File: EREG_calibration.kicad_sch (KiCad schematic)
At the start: 22 parts, among them T1 Low pressure water tank, T2 High pressure COTS tank

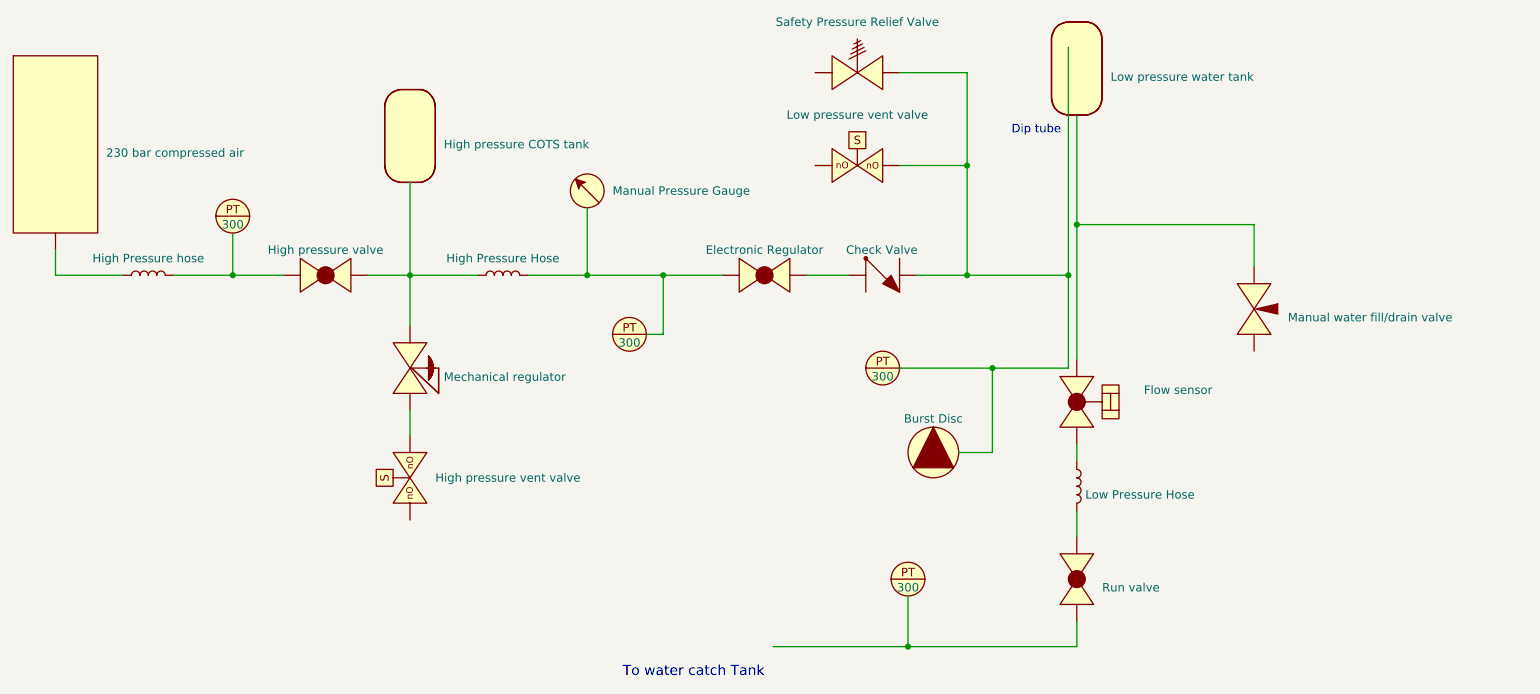
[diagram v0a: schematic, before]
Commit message: more silwood stuff
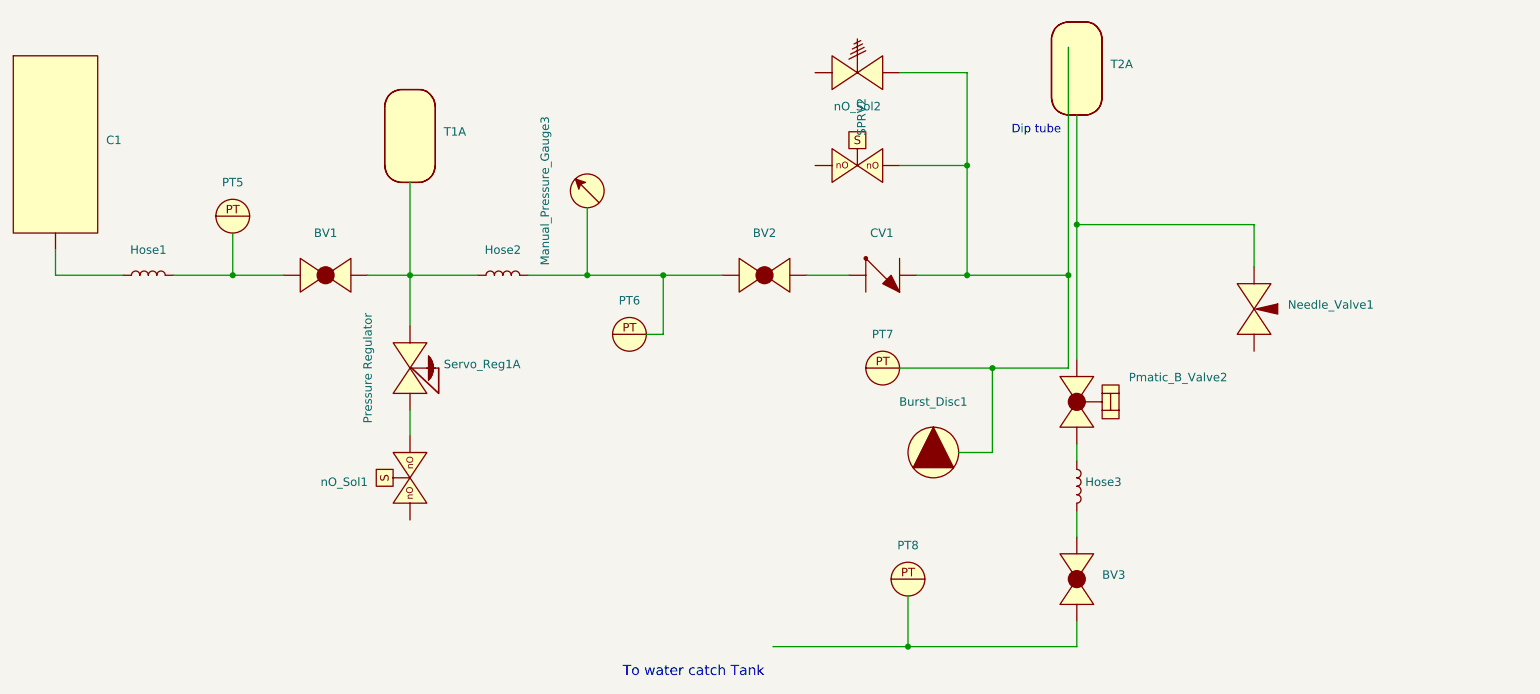
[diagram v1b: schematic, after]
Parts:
- renumbered H1 to Hose1, H2 to Hose2, H3 to Hose3, PT1 to PT5, PT2 to PT6, PT3 to PT7, PT4 to PT8, Pmatic_B_Valve1 to Pmatic_B_Valve2, Reg1 to Servo_Reg1, T2 to T1, T1 to T2, nO_Sol2 to nO_Sol1, nO_Sol1 to nO_Sol2
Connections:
- net at nO_Sol2.: now also Burst_Disc1., CV1., PT7., SPRV2.
- net at Needle_Valve1.: now also Pmatic_B_Valve2., T2.
- net at PT8.: now also BV3.
- net at BV3.: now also Hose3.; no longer PT8.
- net at Pmatic_B_Valve2.: no longer Hose3.
- net at Manual_Pressure_Gauge3.: now also BV2., Hose2., PT6.
- new net: BV1., Hose2., Servo_Reg1., T1.
- new net: BV1., Hose1., PT5.
- new net: Hose3., Pmatic_B_Valve2.
- now unconnected: Burst_Disc1., PT5., PT6., PT7., Pmatic_B_Valve2., SPRV2., T1., T2.

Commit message: Formatiing
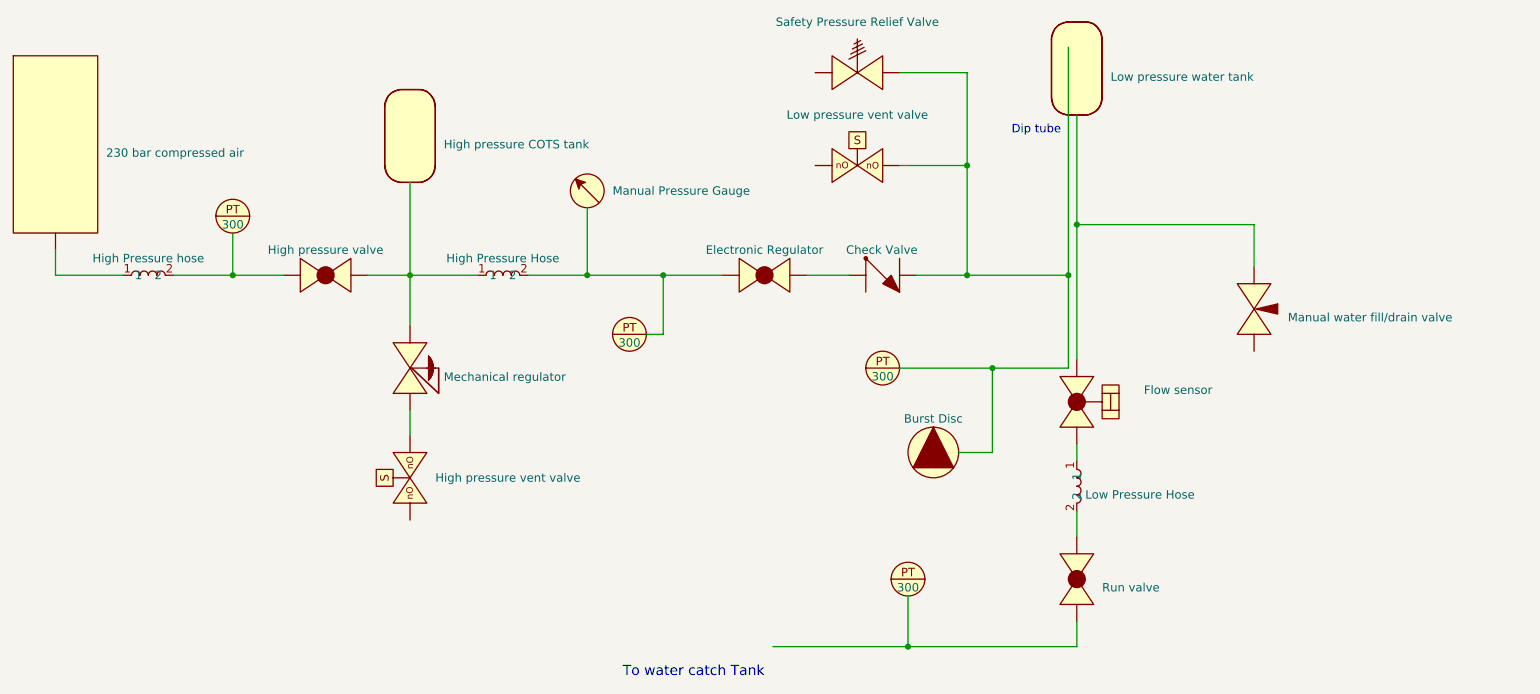
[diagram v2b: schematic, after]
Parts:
- renumbered BV1 to BV69, BV2 to BV70, BV3 to BV71, Burst_Disc1 to Burst_Disc28, C1 to C2, CV1 to CV72, Hose1 to H12, Hose2 to H13, Hose3 to H14, Manual_Pressure_Gauge3 to Manual_Pressure_Gauge13, Needle_Valve1 to Needle_Valve20, PT5 to PT119, PT6 to PT120, PT7 to PT121, PT8 to PT122, Pmatic_B_Valve2 to Pmatic_B_Valve5, Servo_Reg1 to Reg28, SPRV2 to SPRV39, T1 to T25, T2 to T26, nO_Sol1 to nO_Sol45, nO_Sol2 to nO_Sol46
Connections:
- net at nO_Sol46.: now also Burst_Disc28., CV72., PT121., SPRV39.
- net at Needle_Valve20.: now also Pmatic_B_Valve5., T26.
- net at PT122.: now also BV71.
- net at BV71.: now also H14.2; no longer PT122.
- net at Pmatic_B_Valve5.: no longer H14.
- net at Manual_Pressure_Gauge13.: now also BV70., H13.2, PT120.
- net at C2.: now also H12.1; no longer H12.
- new net: BV69., H13.1, Reg28., T25.
- new net: BV69., H12.2, PT119.
- new net: H14.1, Pmatic_B_Valve5.
- now unconnected: Burst_Disc28., PT119., PT120., PT121., Pmatic_B_Valve5., SPRV39., T25., T26.
